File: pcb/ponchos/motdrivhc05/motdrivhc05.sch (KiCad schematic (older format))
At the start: 25 parts, among them J1 MPower, J2 Screw_Terminal_1x04, J3 GW-040, J4 CONN_01X02, Q1 TIP31, Q2 TIP31, U1 L293

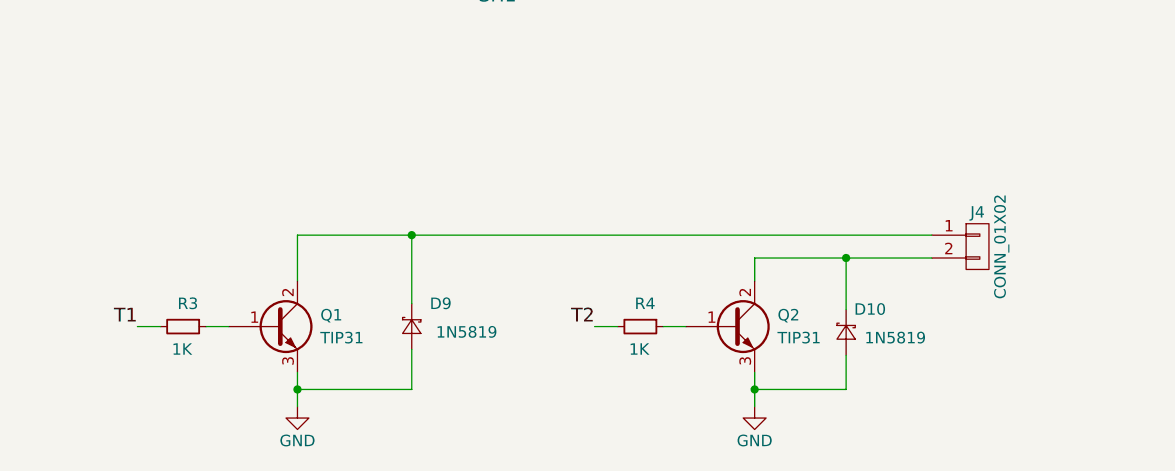
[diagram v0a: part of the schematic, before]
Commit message: En proceso...
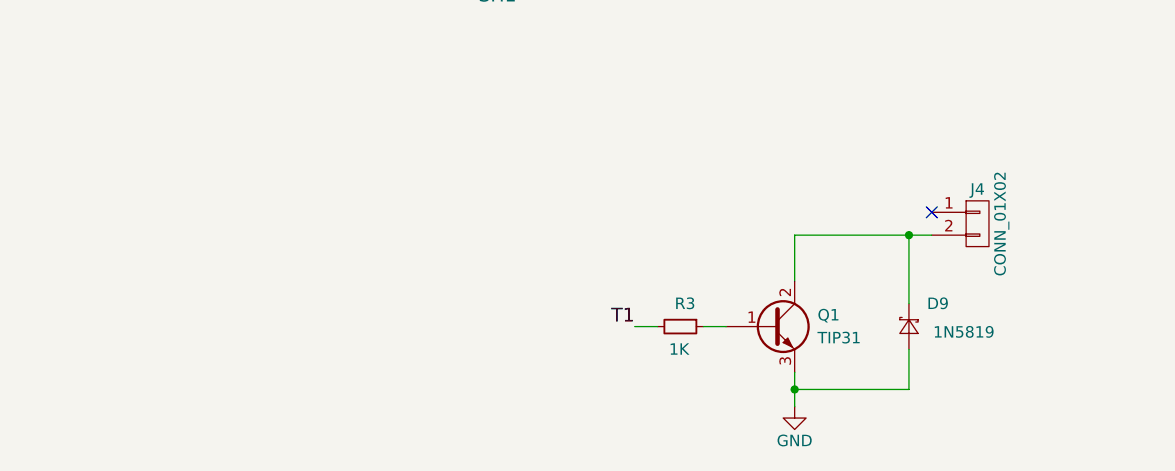
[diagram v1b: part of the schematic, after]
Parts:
- removed D10: 1N5819, Diodes_ThroughHole:Diode_DO-41_SOD81_Horizontal_RM10, symbol D_Schottky_Small
- removed Q2: TIP31, TO_SOT_Packages_THT:TO-220_Neutral123_Horizontal_LargePads, symbol Q_NPN_BCE
- removed R4: 1K, Resistors_ThroughHole:Resistor_Horizontal_RM10mm, symbol R_Small
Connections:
- net at D9.1 (K), Q1.2 (C): now also J4.2 (P2); no longer J4.1 (P1)
- no-connect marks 16 -> 17
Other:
- moved on the sheet: D9, J4, Q1, R3
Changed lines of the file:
@@
 L Q_NPN_BCE Q1
 U 1 1 59A1BF0C
-P 2300 6175
-F 0 "Q1" H 2500 6225 50  0000 L CNN
-F 1 "TIP31" H 2500 6125 50  0000 L CNN
-F 2 "TO_SOT_Packages_THT:TO-220_Neutral123_Horizontal_LargePads" H 2500 6275 50  0001 C CNN
-F 3 "" H 2300 6175 50  0001 C CNN
-	1    2300 6175
+P 4475 6175
+F 0 "Q1" H 4675 6225 50  0000 L CNN
+F 1 "TIP31" H 4675 6125 50  0000 L CNN
+F 2 "TO_SOT_Packages_THT:TO-220_Neutral123_Horizontal_LargePads" H 4675 6275 50  0001 C CNN
+F 3 "" H 4475 6175 50  0001 C CNN
+	1    4475 6175
 	1    0    0    -1
 $EndComp
@@
 L GND #PWR014
 U 1 1 59A1C2CB
-P 2400 6525
-F 0 "#PWR014" H 2400 6275 50  0001 C CNN
-F 1 "GND" H 2400 6375 50  0000 C CNN
-F 2 "" H 2400 6525 50  0001 C CNN
-F 3 "" H 2400 6525 50  0001 C CNN
-	1    2400 6525
-	1    0    0    -1
-$EndComp
-Wire Wire Line
-	2400 6375 2400 6525
-$Comp
-L Q_NPN_BCE Q2
-U 1 1 59A1C711
-P 4300 6175
-F 0 "Q2" H 4500 6225 50  0000 L CNN
-F 1 "TIP31" H 4500 6125 50  0000 L CNN
-F 2 "TO_SOT_Packages_THT:TO-220_Neutral123_Horizontal_LargePads" H 4500 6275 50  0001 C CNN
-F 3 "" H 4300 6175 50  0001 C CNN
-	1    4300 6175
-	1    0    0    -1
-$EndComp
-$Comp
-L GND #PWR015
-U 1 1 59A1C717
-P 4400 6525
-F 0 "#PWR015" H 4400 6275 50  0001 C CNN
-F 1 "GND" H 4400 6375 50  0000 C CNN
-F 2 "" H 4400 6525 50  0001 C CNN
-F 3 "" H 4400 6525 50  0001 C CNN
-	1    4400 6525
-	1    0    0    -1
-$EndComp
-Wire Wire Line
-	4400 6375 4400 6525
-Text Label 3700 6175 2    60   ~ 0
-T2
-Wire Wire Line
-	3800 6175 3700 6175
+P 4575 6525
+F 0 "#PWR014" H 4575 6275 50  0001 C CNN
+F 1 "GND" H 4575 6375 50  0000 C CNN
+F 2 "" H 4575 6525 50  0001 C CNN
+F 3 "" H 4575 6525 50  0001 C CNN
+	1    4575 6525
+	1    0    0    -1
+$EndComp
+Wire Wire Line
+	4575 6375 4575 6525
 $Comp
 L CONN_01X02 J4
 U 1 1 59A1C921
-P 5375 5825
-F 0 "J4" H 5375 5975 50  0000 C CNN
-F 1 "CONN_01X02" V 5475 5825 50  0000 C CNN
-F 2 "Pin_Headers:Pin_Header_Straight_1x02" H 5375 5825 50  0001 C CNN
-F 3 "" H 5375 5825 50  0001 C CNN
-	1    5375 5825
-	1    0    0    -1
-$EndComp
-Wire Wire Line
-	2400 5775 5175 5775
-Wire Wire Line
-	2400 5775 2400 5975
-Wire Wire Line
-	4400 5875 5175 5875
-Wire Wire Line
-	4400 5875 4400 5975
-$Comp
-L R_Small R4
-U 1 1 59A1CD6A
-P 3900 6175
-F 0 "R4" V 3800 6150 50  0000 L CNN
-F 1 "1K" V 4000 6125 50  0000 L CNN
-F 2 "Resistors_ThroughHole:Resistor_Horizontal_RM10mm" H 3900 6175 50  0001 C CNN
-F 3 "" H 3900 6175 50  0001 C CNN
-	1    3900 6175
-	0    1    1    0
-$EndComp
-Wire Wire Line
-	4100 6175 4000 6175
-Text Label 1700 6175 2    60   ~ 0
+P 5375 5725
+F 0 "J4" H 5375 5875 50  0000 C CNN
+F 1 "CONN_01X02" V 5475 5725 50  0000 C CNN
+F 2 "Pin_Headers:Pin_Header_Straight_1x02" H 5375 5725 50  0001 C CNN
+F 3 "" H 5375 5725 50  0001 C CNN
+	1    5375 5725
+	1    0    0    -1
+$EndComp
+Wire Wire Line
+	4575 5775 5175 5775
+Wire Wire Line
+	4575 5775 4575 5975
+Text Label 3875 6175 2    60   ~ 0
 T1
 Wire Wire Line
-	1800 6175 1700 6175
+	3975 6175 3875 6175
 $Comp
 L R_Small R3
 U 1 1 59A1D20C
-P 1900 6175
-F 0 "R3" V 1800 6150 50  0000 L CNN
-F 1 "1K" V 2000 6125 50  0000 L CNN
-F 2 "Resistors_ThroughHole:Resistor_Horizontal_RM10mm" H 1900 6175 50  0001 C CNN
-F 3 "" H 1900 6175 50  0001 C CNN
-	1    1900 6175
+P 4075 6175
+F 0 "R3" V 3975 6150 50  0000 L CNN
+F 1 "1K" V 4175 6125 50  0000 L CNN
+F 2 "Resistors_ThroughHole:Resistor_Horizontal_RM10mm" H 4075 6175 50  0001 C CNN
+F 3 "" H 4075 6175 50  0001 C CNN
+	1    4075 6175
 	0    1    1    0
 $EndComp
 Wire Wire Line
-	2100 6175 2000 6175
+	4275 6175 4175 6175
 $Comp
 L D_Schottky_Small D9
 U 1 1 59A1D6C4
-P 2900 6175
-F 0 "D9" V 2800 6000 50  0000 L CNN
-F 1 "1N5819" V 2925 5800 50  0000 L CNN
-F 2 "Diodes_ThroughHole:Diode_DO-41_SOD81_Horizontal_RM10" V 2900 6175 50  0001 C CNN
-F 3 "" V 2900 6175 50  0001 C CNN
-	1    2900 6175
-	0    -1   1    0
-$EndComp
-$Comp
-L D_Schottky_Small D10
-U 1 1 59A1D6CA
-P 4800 6200
-F 0 "D10" V 4700 6025 50  0000 L CNN
-F 1 "1N5819" V 4825 5850 50  0000 L CNN
-F 2 "Diodes_ThroughHole:Diode_DO-41_SOD81_Horizontal_RM10" V 4800 6200 50  0001 C CNN
-F 3 "" V 4800 6200 50  0001 C CNN
-	1    4800 6200
-	0    -1   1    0
-$EndComp
-Wire Wire Line
-	4800 5875 4800 6100
-Connection ~ 4800 5875
-Wire Wire Line
-	4800 6300 4800 6450
-Wire Wire Line
-	4800 6450 4400 6450
-Connection ~ 4400 6450
-Wire Wire Line
-	2900 6075 2900 5775
-Connection ~ 2900 5775
-Wire Wire Line
-	2900 6275 2900 6450
-Wire Wire Line
-	2900 6450 2400 6450
-Connection ~ 2400 6450
+P 5075 6175
+F 0 "D9" V 4975 6000 50  0000 L CNN
+F 1 "1N5819" V 5100 5800 50  0000 L CNN
+F 2 "Diodes_ThroughHole:Diode_DO-41_SOD81_Horizontal_RM10" V 5075 6175 50  0001 C CNN
+F 3 "" V 5075 6175 50  0001 C CNN
+	1    5075 6175
+	0    -1   1    0
+$EndComp
+Wire Wire Line
+	5075 6075 5075 5775
+Connection ~ 5075 5775
+Wire Wire Line
+	5075 6275 5075 6450
+Wire Wire Line
+	5075 6450 4575 6450
+Connection ~ 4575 6450
 Text Label 4150 2450 0    60   ~ 0
 T1
@@
 $EndComp
 $Comp
-L GND #PWR016
+L GND #PWR015
 U 1 1 59A4C1EF
 P 7850 5400
-F 0 "#PWR016" H 7850 5150 50  0001 C CNN
+F 0 "#PWR015" H 7850 5150 50  0001 C CNN
 F 1 "GND" H 7850 5250 50  0000 C CNN
 F 2 "" H 7850 5400 50  0001 C CNN
@@
 	7850 4675 7725 4675
 $Comp
-L GND #PWR017
+L GND #PWR016
 U 1 1 59A4C3C7
 P 8700 5350
-F 0 "#PWR017" H 8700 5100 50  0001 C CNN
+F 0 "#PWR016" H 8700 5100 50  0001 C CNN
 F 1 "GND" H 8700 5200 50  0000 C CNN
 F 2 "" H 8700 5350 50  0001 C CNN
@@
 	8700 5200 8700 5350
 $Comp
-L +5V #PWR018
+L +5V #PWR017
 U 1 1 59A4C522
 P 8800 4575
-F 0 "#PWR018" H 8800 4425 50  0001 C CNN
+F 0 "#PWR017" H 8800 4425 50  0001 C CNN
 F 1 "+5V" H 8800 4715 50  0000 C CNN
 F 2 "" H 8800 4575 50  0001 C CNN
@@
 NoConn ~ 2500 4550
 $Comp
-L PWR_FLAG #FLG019
+L PWR_FLAG #FLG018
 U 1 1 59A5033C
 P 2025 1175
-F 0 "#FLG019" H 2025 1250 50  0001 C CNN
+F 0 "#FLG018" H 2025 1250 50  0001 C CNN
 F 1 "PWR_FLAG" H 2025 1325 50  0000 C CNN
 F 2 "" H 2025 1175 50  0001 C CNN
@@
 $EndComp
 $Comp
-L PWR_FLAG #FLG020
+L PWR_FLAG #FLG019
 U 1 1 59A503B2
 P 2650 1375
-F 0 "#FLG020" H 2650 1450 50  0001 C CNN
+F 0 "#FLG019" H 2650 1450 50  0001 C CNN
 F 1 "PWR_FLAG" H 2650 1525 50  0000 C CNN
 F 2 "" H 2650 1375 50  0001 C CNN
@@
 Wire Wire Line
 	7625 3000 7475 3000
+NoConn ~ 5175 5675
 $EndSCHEMATC

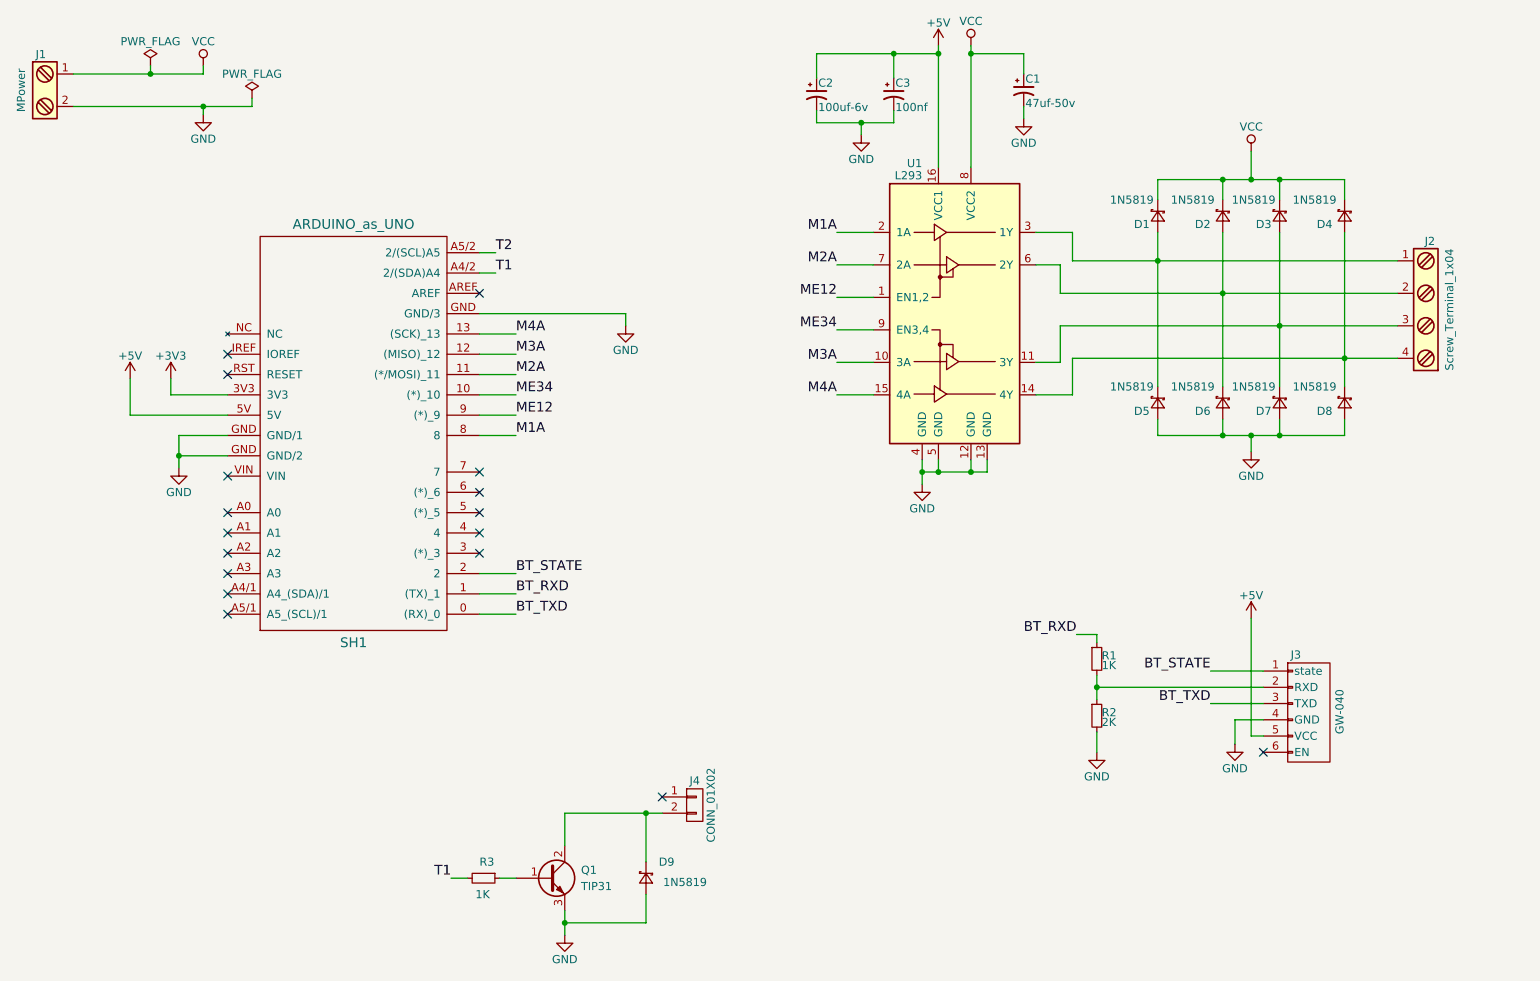
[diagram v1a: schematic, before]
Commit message: En processo...
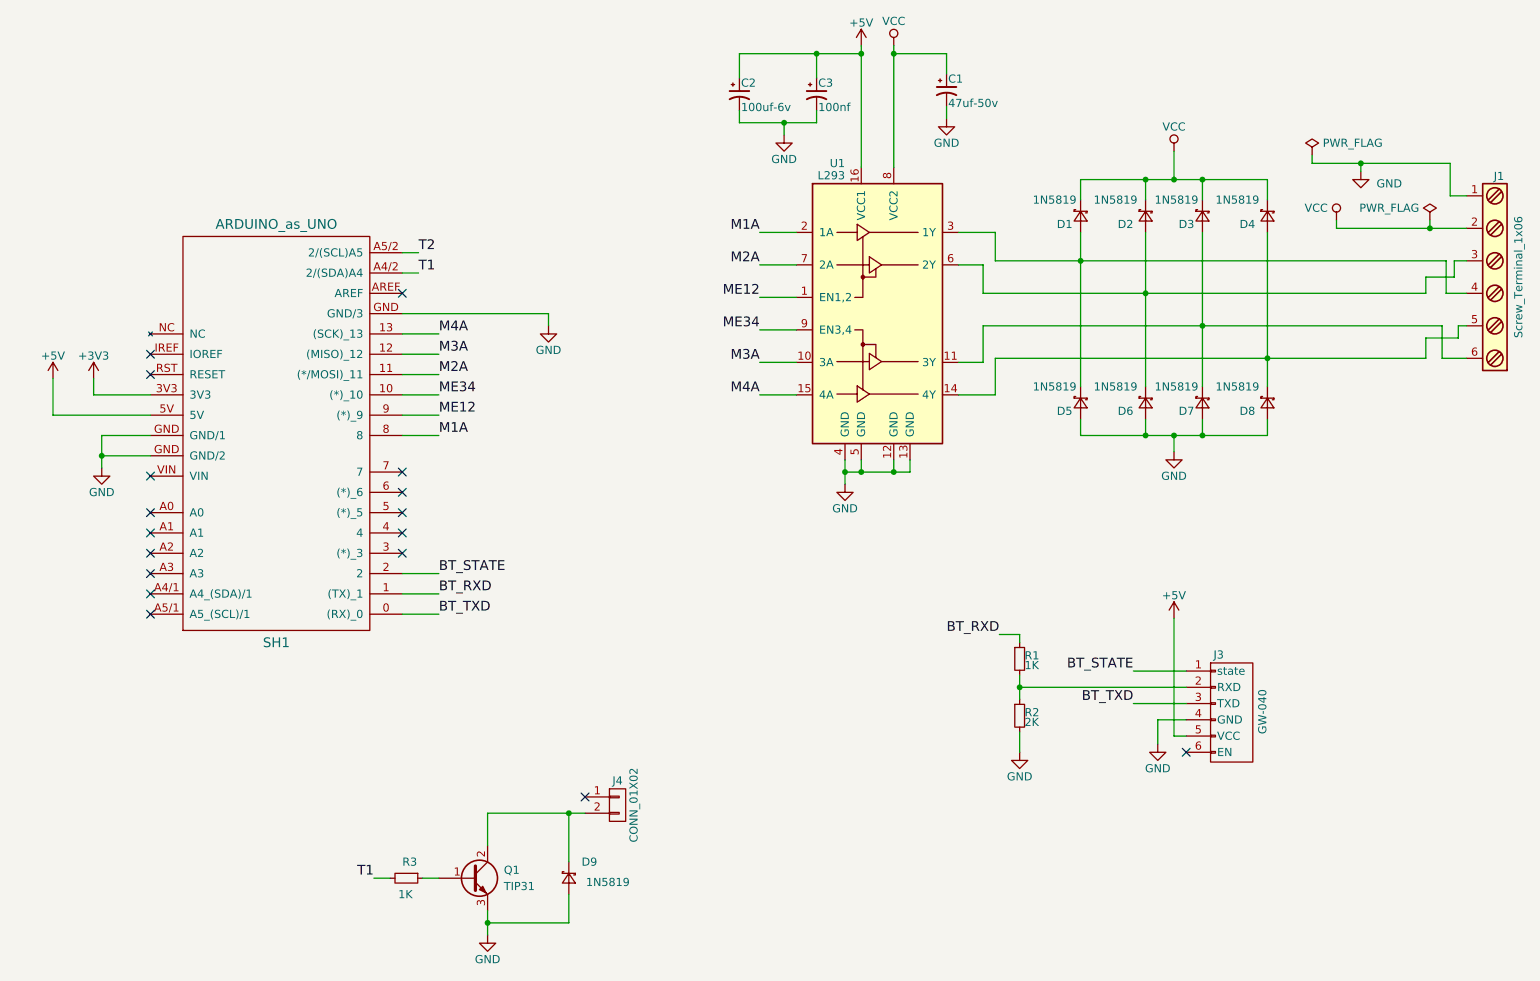
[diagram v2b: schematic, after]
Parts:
- removed J1: MPower, Connect:bornier2, symbol Screw_Terminal_1x02
- removed J2: Screw_Terminal_1x04, Connect:bornier4, symbol Screw_Terminal_1x04
- added J1: Screw_Terminal_1x06, Terminal_Blocks:TerminalBlock_Pheonix_MKDS1.5-6pol, symbol Screw_Terminal_1x06
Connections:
- net GND: now also J1.1
- net VCC: now also J1.2
- net at D1.2 (A), D5.1 (K), U1.3 (1Y): now also J1.4
- net at D2.2 (A), D6.1 (K), U1.6 (2Y): now also J1.3
- net at D3.2 (A), D7.1 (K), U1.11 (3Y): now also J1.6
- net at D4.2 (A), D8.1 (K), U1.14 (4Y): now also J1.5
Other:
- moved on the sheet: C1, C2, C3, D1, D2, D3, D4, D5, D6, D7, D8, D9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
